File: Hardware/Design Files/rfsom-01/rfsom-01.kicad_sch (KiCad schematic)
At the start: 2 parts, among them J1 TC2050

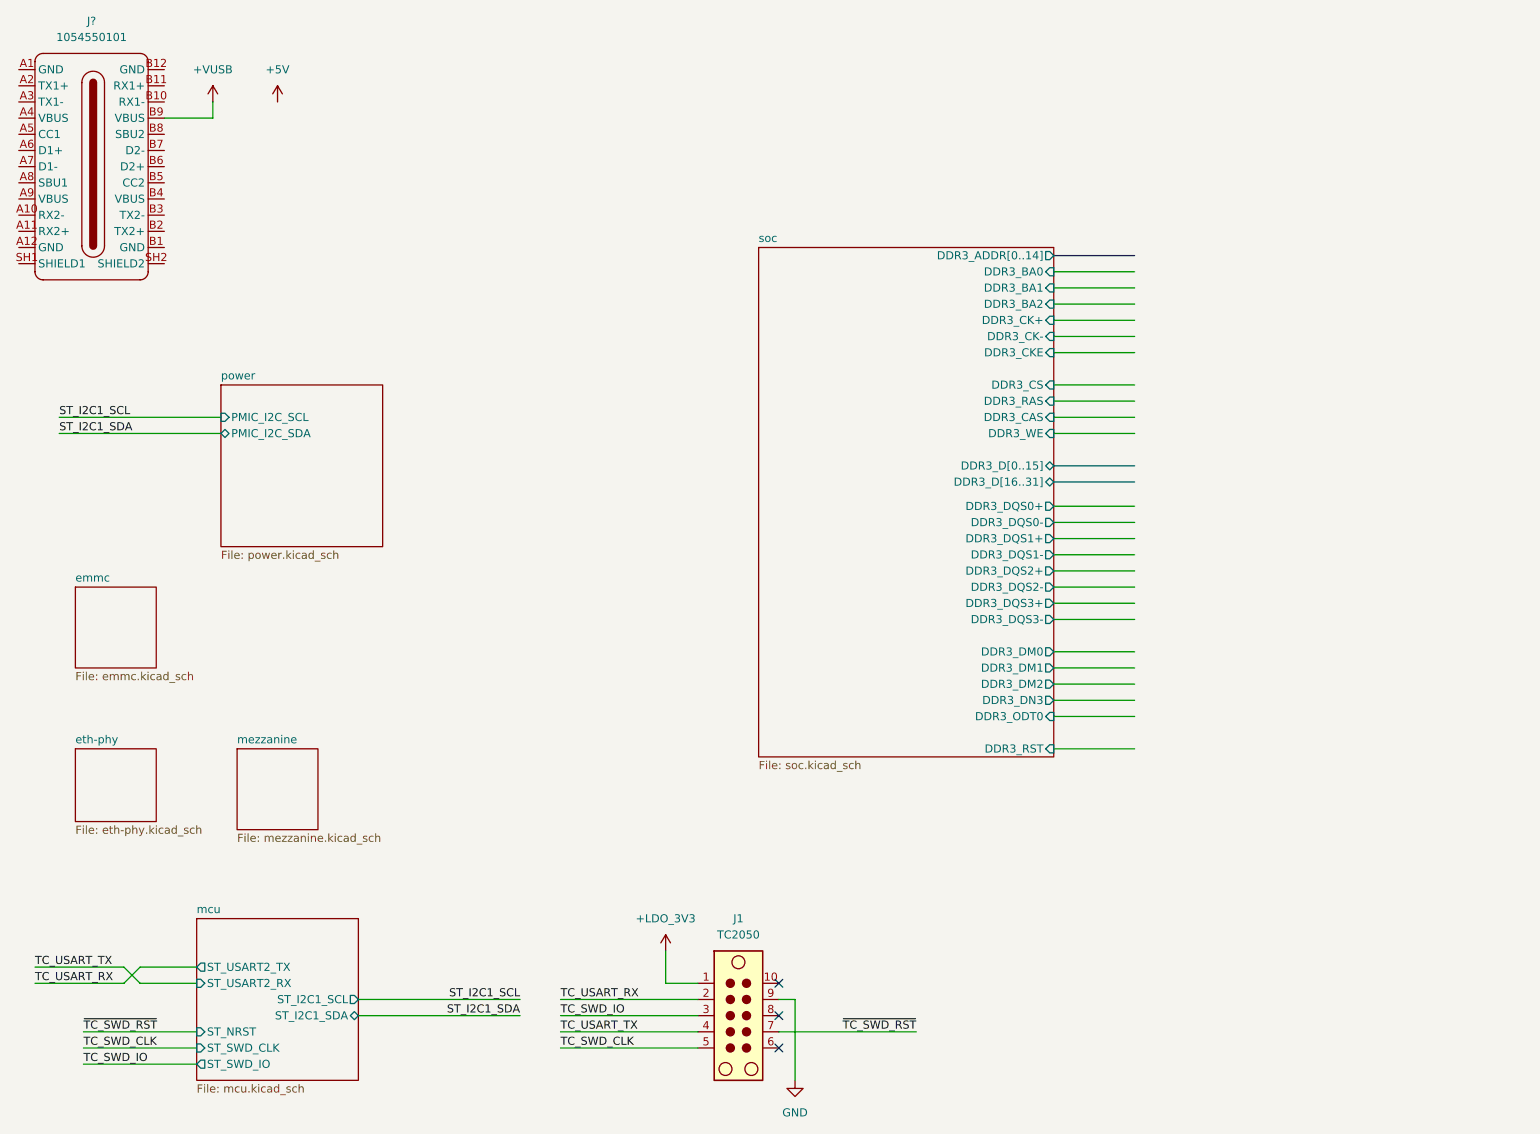
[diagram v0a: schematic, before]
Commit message: ps progress; added ftdi; mezz pinout pedinging;
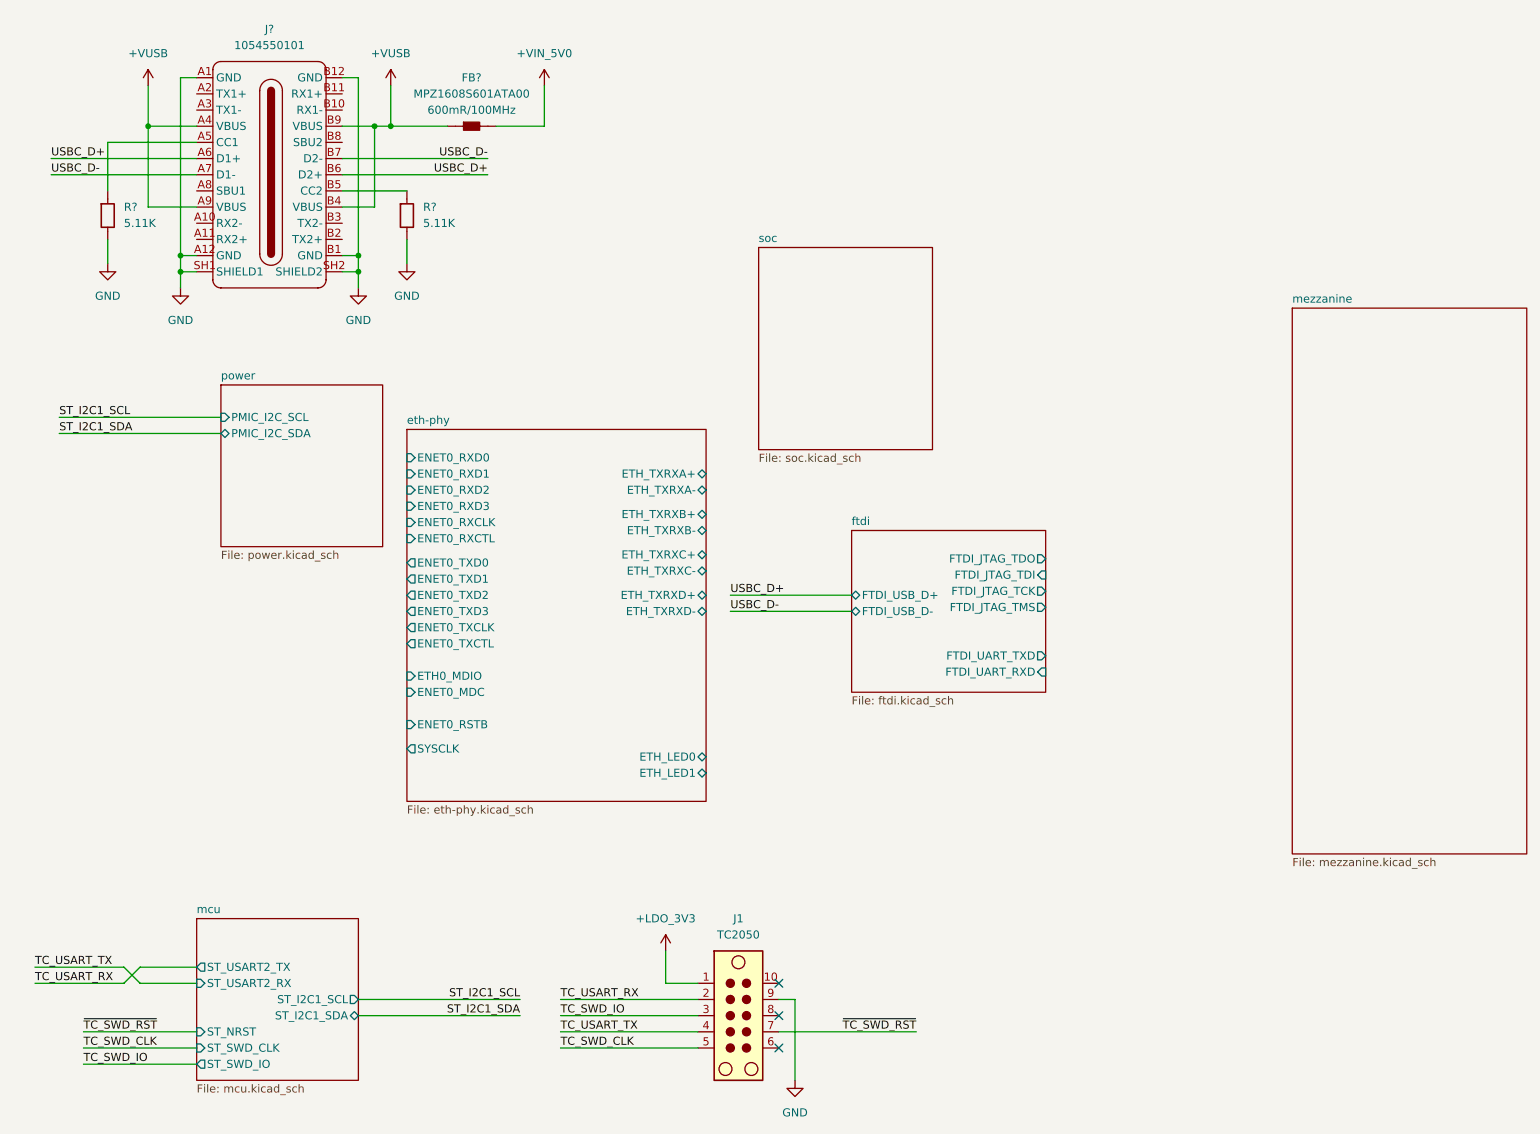
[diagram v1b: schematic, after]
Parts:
- added FB?: MPZ1608S601ATA00, Resistor_SMD:R_0603_1608Metric, symbol Inductors:MPZ1608S601ATA00
- added R? (x2): RC0603FR-135K11L, Resistor_SMD:R_0603_1608Metric, symbol Resistors:RC0603FR-135K11L
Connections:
- net +VUSB: now also J?.A4 (VBUS), J?.A9 (VBUS), J?.B4 (VBUS), FB?.1
- net GND: now also J?.A1 (GND), J?.A12 (GND), J?.B1 (GND), J?.B12 (GND), J?.SH1 (SHIELD1), J?.SH2 (SHIELD2), R?.2, R?.2
- net at J?.A5 (CC1): now also R?.1
- net USBC_D+: now reaches J?.A6 (D1+)
- net USBC_D+: now also J?.B6 (D2+)
- net USBC_D-: now reaches J?.A7 (D1-)
- net USBC_D-: now also J?.B7 (D2-)
- net at J?.B5 (CC2): now also R?.1
- new net +VIN_5V0: FB?.2
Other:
- removed sheet emmc
- added sheet ftdi (ftdi.kicad_sch)
- sheet eth-phy ports: added ENET0_MDC, ENET0_RSTB, ENET0_RXCLK, ENET0_RXCTL, ENET0_RXD0, ENET0_RXD1, ENET0_RXD2, ENET0_RXD3, ENET0_TXCLK, ENET0_TXCTL, ENET0_TXD0, ENET0_TXD1, ENET0_TXD2, ENET0_TXD3, ETH0_MDIO, ETH_LED0, ETH_LED1, ETH_TXRXA+, ETH_TXRXA-, ETH_TXRXB+, ETH_TXRXB-, ETH_TXRXC+, ETH_TXRXC-, ETH_TXRXD+, ETH_TXRXD-, SYSCLK; removed none
- sheet soc ports: added none; removed DDR3_ADDR[0..14], DDR3_BA0, DDR3_BA1, DDR3_BA2, DDR3_CAS, DDR3_CK+, DDR3_CK-, DDR3_CKE, DDR3_CS, DDR3_DM0, DDR3_DM1, DDR3_DM2, DDR3_DN3, DDR3_DQS0+, DDR3_DQS0-, DDR3_DQS1+, DDR3_DQS1-, DDR3_DQS2+, DDR3_DQS2-, DDR3_DQS3+, DDR3_DQS3-, DDR3_D[0..15], DDR3_D[16..31], DDR3_ODT0, DDR3_RAS, DDR3_RST, DDR3_WE
- moved on the sheet: J?
